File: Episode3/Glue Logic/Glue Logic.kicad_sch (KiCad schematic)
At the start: 5 parts, among them J1 5V DC

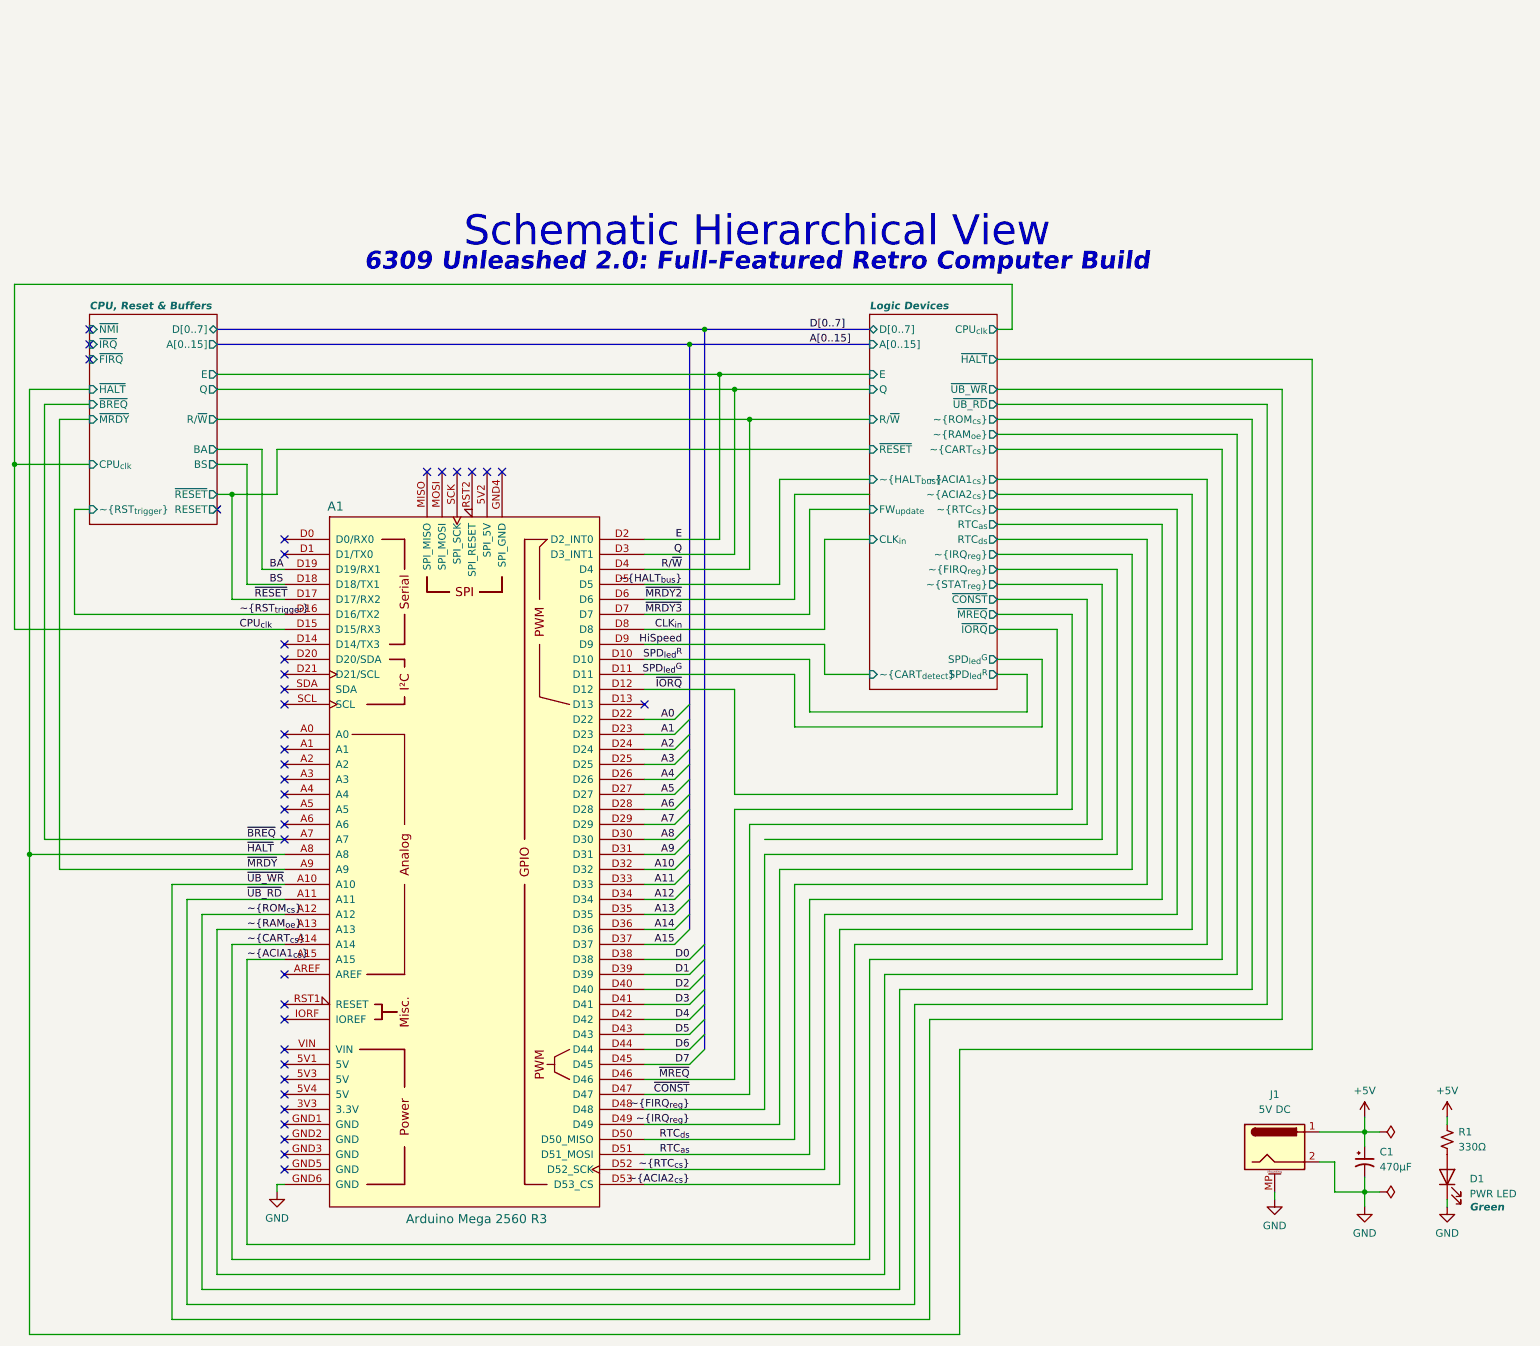
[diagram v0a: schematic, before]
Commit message: Pushing back everything, due to PC reinstall.
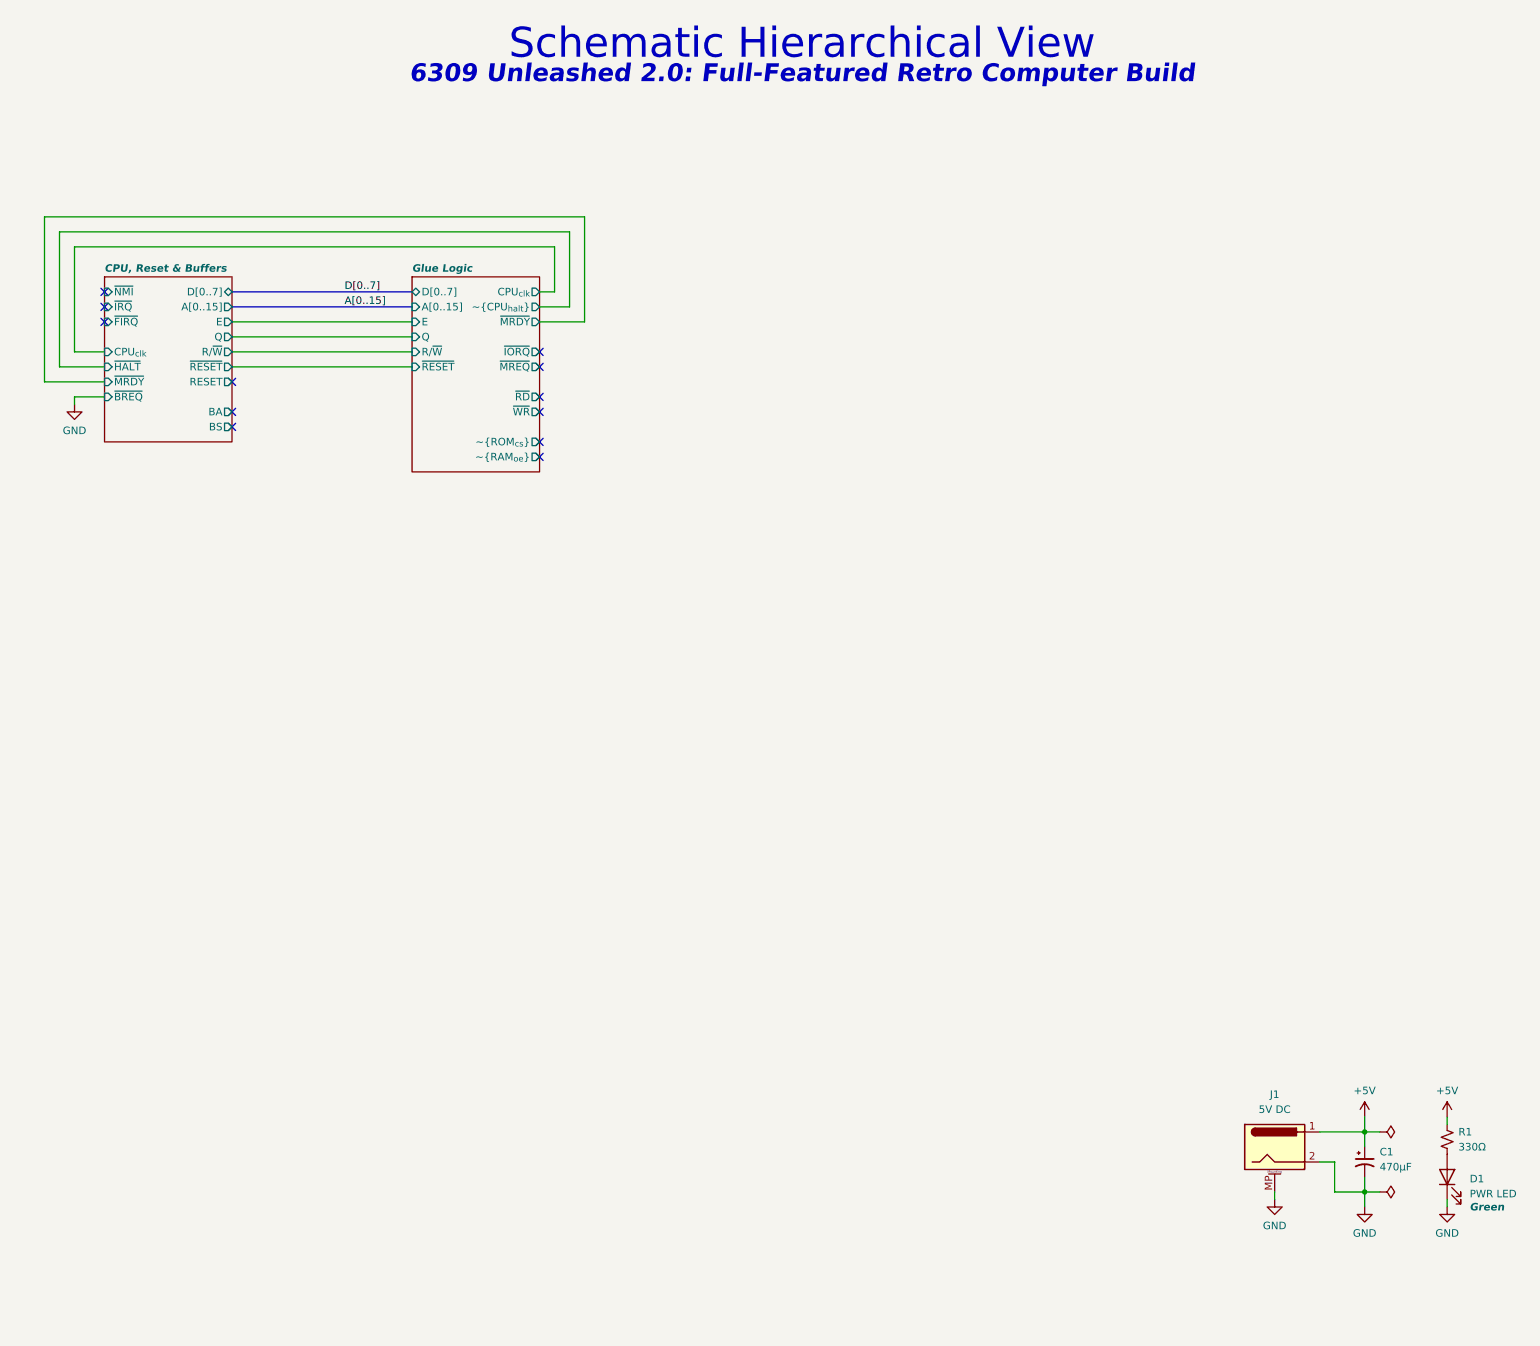
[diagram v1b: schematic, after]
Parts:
- removed A1: Arduino Mega 2560 R3, symbol 6309 v2.0:Arduino_Mega2560_R3_Shield
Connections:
- no-connect marks 38 -> 12
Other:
- sheet Logic Devices renamed Glue Logic
- sheet CPU, Reset & Buffers ports: added none; removed ~{RST_{trigger}}
- sheet Glue Logic: file PLD.kicad_sch -> Glue.kicad_sch
- sheet Glue Logic ports: added ~{CPU_{halt}}, ~{MRDY}, ~{RD}, ~{WR}; removed CLK_{in}, FW_{update}, RTC_{as}, RTC_{ds}, SPD_{led}^{G}, SPD_{led}^{R}, ~{ACIA1_{cs}}, ~{ACIA2_{cs}}, ~{CART_{cs}}, ~{CART_{detect}}, ~{CONST}, ~{FIRQ_{reg}}, ~{HALT_{bus}}, ~{HALT}, ~{IRQ_{reg}}, ~{RTC_{cs}}, ~{STAT_{reg}}, ~{UB_RD}, ~{UB_WR}

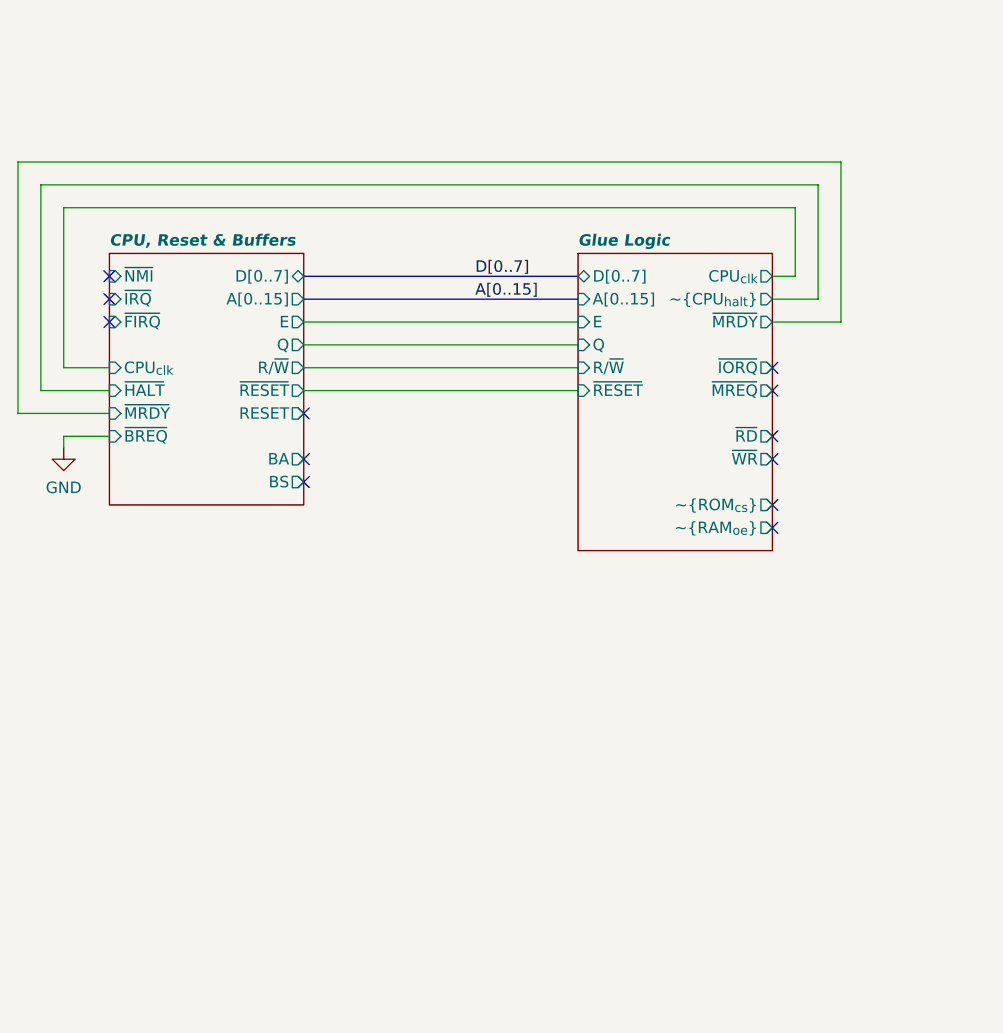
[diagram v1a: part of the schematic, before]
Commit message: Tied up a few loose ends in the PLD page.
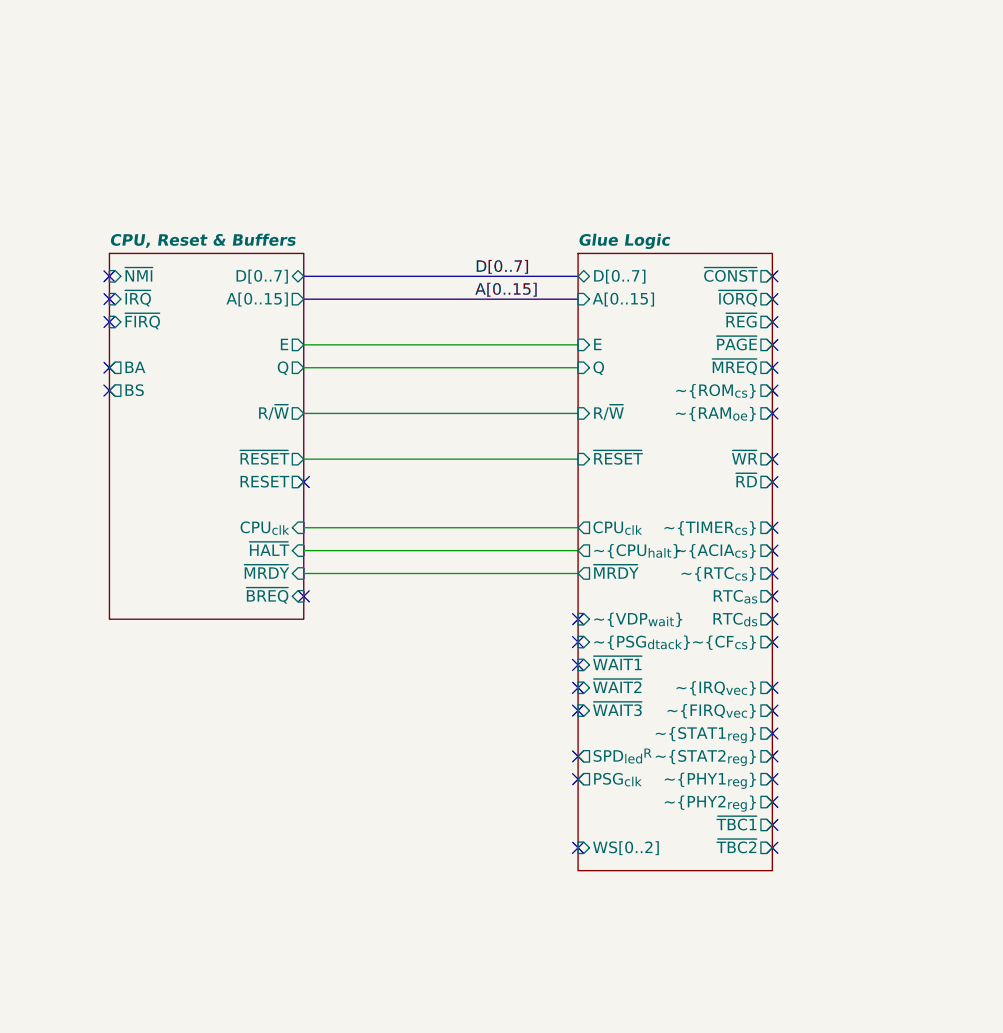
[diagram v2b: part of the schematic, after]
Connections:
- no-connect marks 12 -> 38
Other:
- sheet Glue Logic ports: added PSG_{clk}, RTC_{as}, RTC_{ds}, SPD_{led}^{R}, WS[0..2], ~{ACIA_{cs}}, ~{CF_{cs}}, ~{CONST}, ~{FIRQ_{vec}}, ~{IRQ_{vec}}, ~{PAGE}, ~{PHY1_{reg}}, ~{PHY2_{reg}}, ~{PSG_{dtack}}, ~{REG}, ~{RTC_{cs}}, ~{STAT1_{reg}}, ~{STAT2_{reg}}, ~{TBC1}, ~{TBC2}, ~{TIMER_{cs}}, ~{VDP_{wait}}, ~{WAIT1}, ~{WAIT2}, ~{WAIT3}; removed none
